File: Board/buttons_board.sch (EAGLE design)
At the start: 5 parts, among them U1 TEM-HUM-AM2302(4P-25.0X15.0MM)

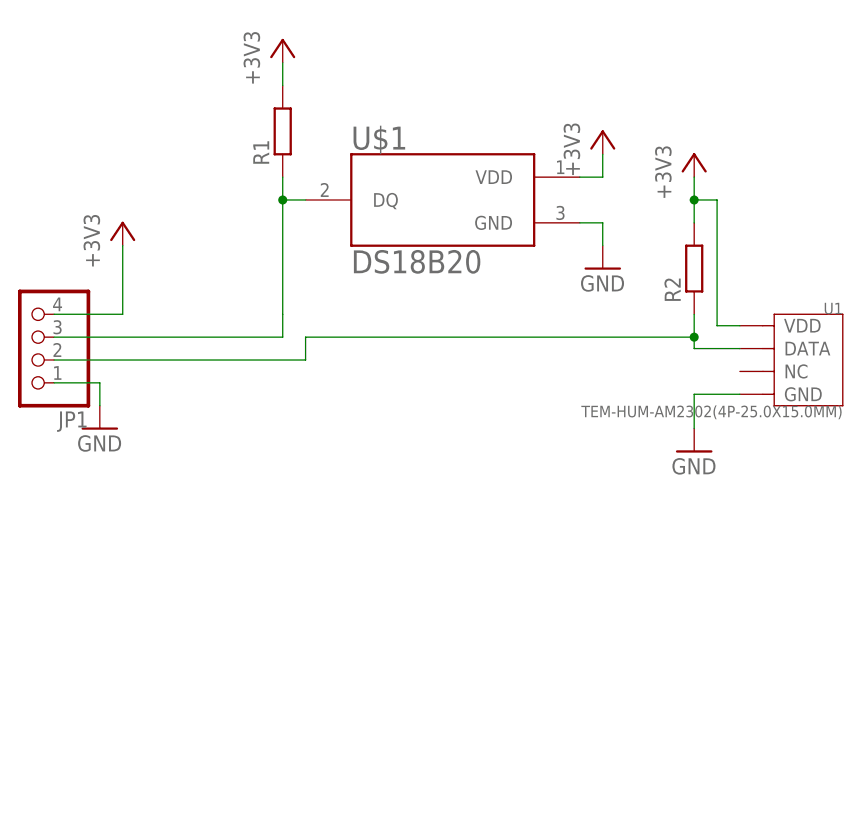
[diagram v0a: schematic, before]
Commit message: Update
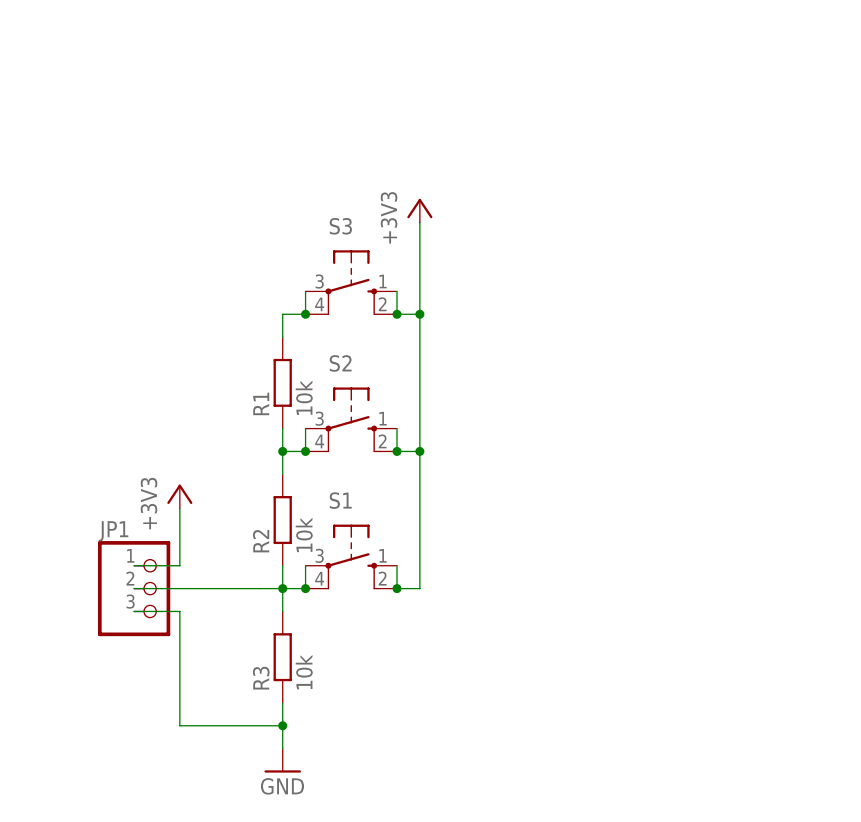
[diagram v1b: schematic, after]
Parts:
- removed U$1: DS18B20, DS18B20_PAR:DS18B20
- removed U1: TEM-HUM-AM2302(4P-25.0X15.0MM), TEM-HUM-AM2302_4P-25.0X15.0MM_:TEM-HUM-AM2302(4P-25.0X15.0MM)
- added R3: 10k, rcl:R-EU_R1206
- added S1, S2, S3: (no value), switch-omron:10-XX
- JP1: device pinhead:PINHD-1X4 -> pinhead:PINHD-1X3/90
- R1, R2: value (none) -> 10k
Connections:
- new net N$3: R1.2, S3.P, S3.P1
- net +3V3: now also JP1.1, S1.S, S1.S1, S2.S, S2.S1, S3.S, S3.S1; no longer JP1.4, R1.2, R2.2, U$1.VDD, U1.VDD
- net GND: now also JP1.3, R3.1; no longer JP1.1, U$1.GND, U1.GND
- net N$1: now also R3.2, S1.P, S1.P1; no longer U1.DATA
- net N$2: now also R2.2, S2.P, S2.P1; no longer JP1.3, U$1.DQ
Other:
- moved on the sheet: R1, R2
